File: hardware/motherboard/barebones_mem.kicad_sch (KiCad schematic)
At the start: 25 parts, among them Q4 MMBT3904, U30 W25Q256JWEIQ, U31 PCF85063ATL/1,118, U71 DRV5032DUDBZR, Y5 ABS07-32.768KHZ-T

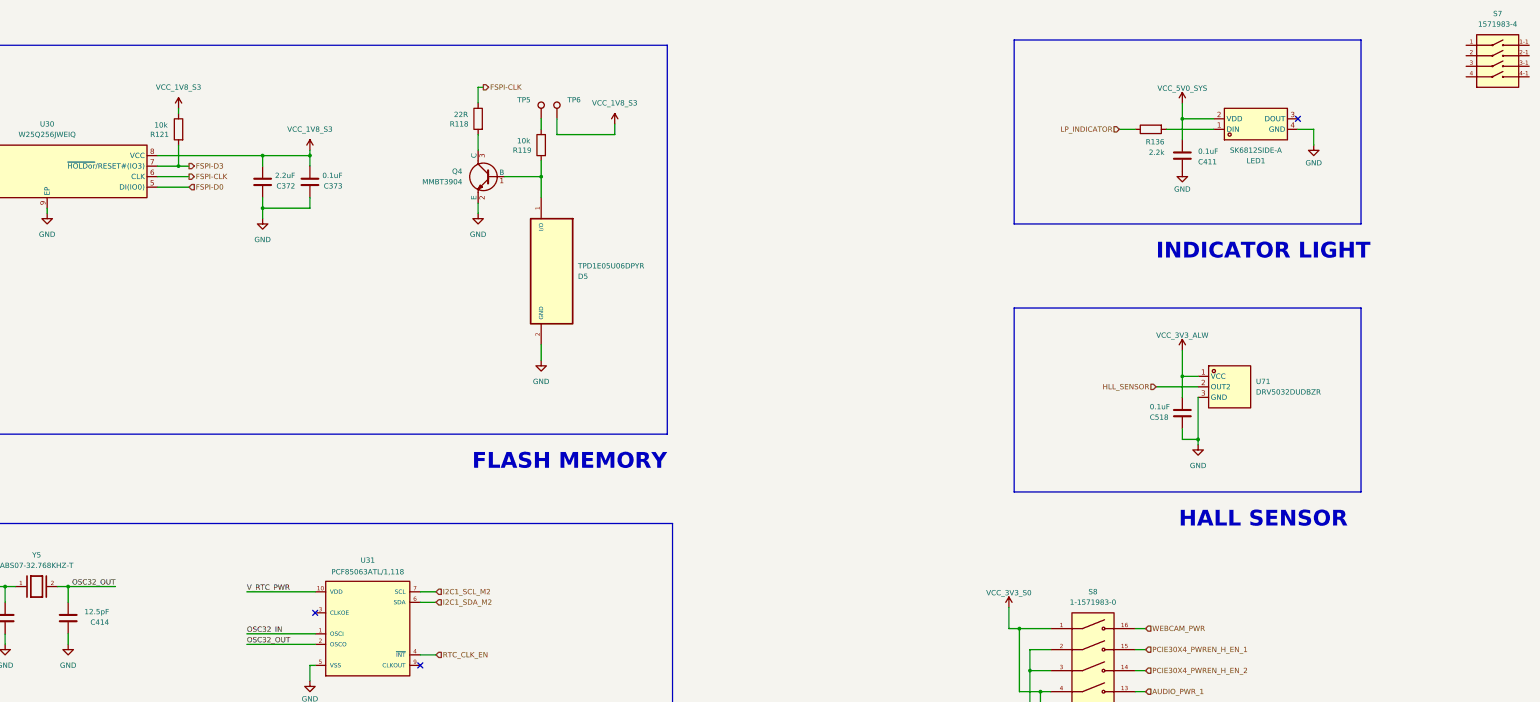
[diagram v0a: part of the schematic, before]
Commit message: started routing on LPDDR4x RAM
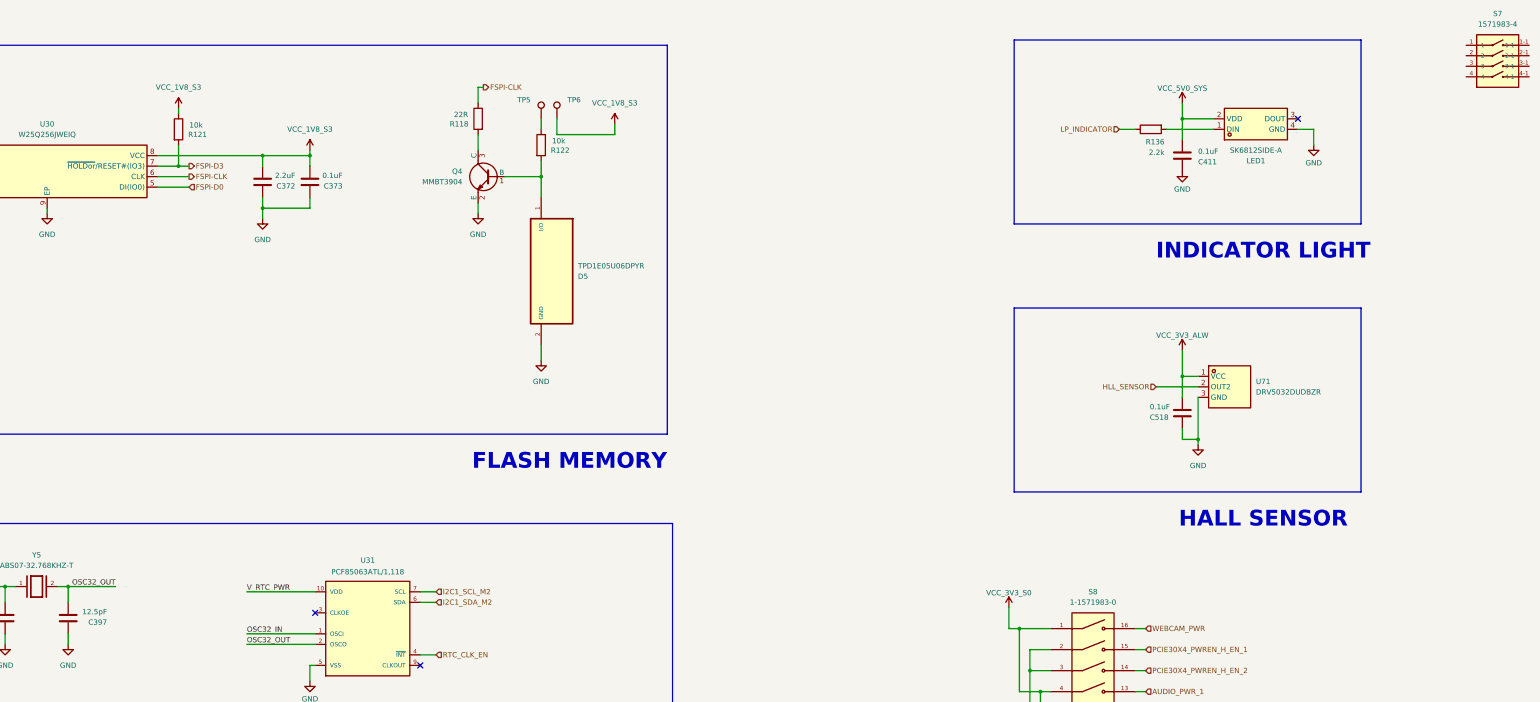
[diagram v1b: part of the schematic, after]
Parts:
- removed C414: 12.5pF, Capacitor_SMD:C_0603_1608Metric, symbol Device:C
- removed R119: 10k, Resistor_SMD:R_0603_1608Metric, symbol Device:R
- added C397: 12.5pF, Capacitor_SMD:C_0402_1005Metric, symbol Device:C
- added R122: 10k, Resistor_SMD:R_0402_1005Metric, symbol Device:R
- C372, C373, C395, C524: footprint Capacitor_SMD:C_0603_1608Metric -> Capacitor_SMD:C_0402_1005Metric
- R118, R120, R121, R212: footprint Resistor_SMD:R_0603_1608Metric -> Resistor_SMD:R_0402_1005Metric
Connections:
- net GND: now also C397.1
- net OSC32_OUT: now also C397.2
- net at D5.1 (I/O), Q4.1 (B): now also R122.2
- net at TP5.1: now also R122.1
